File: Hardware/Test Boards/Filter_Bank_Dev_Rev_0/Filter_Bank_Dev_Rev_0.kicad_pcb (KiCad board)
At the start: 2 copper layers, 50 x 50 mm, 24 parts, among them J1 USB_B_Micro, J2 RF IN, J3 RF OUT, SW1 KAE02LGGR, U1 PE42440, U2 74AHC1G04, U3 AMS1117-3.3, U4 PE42440

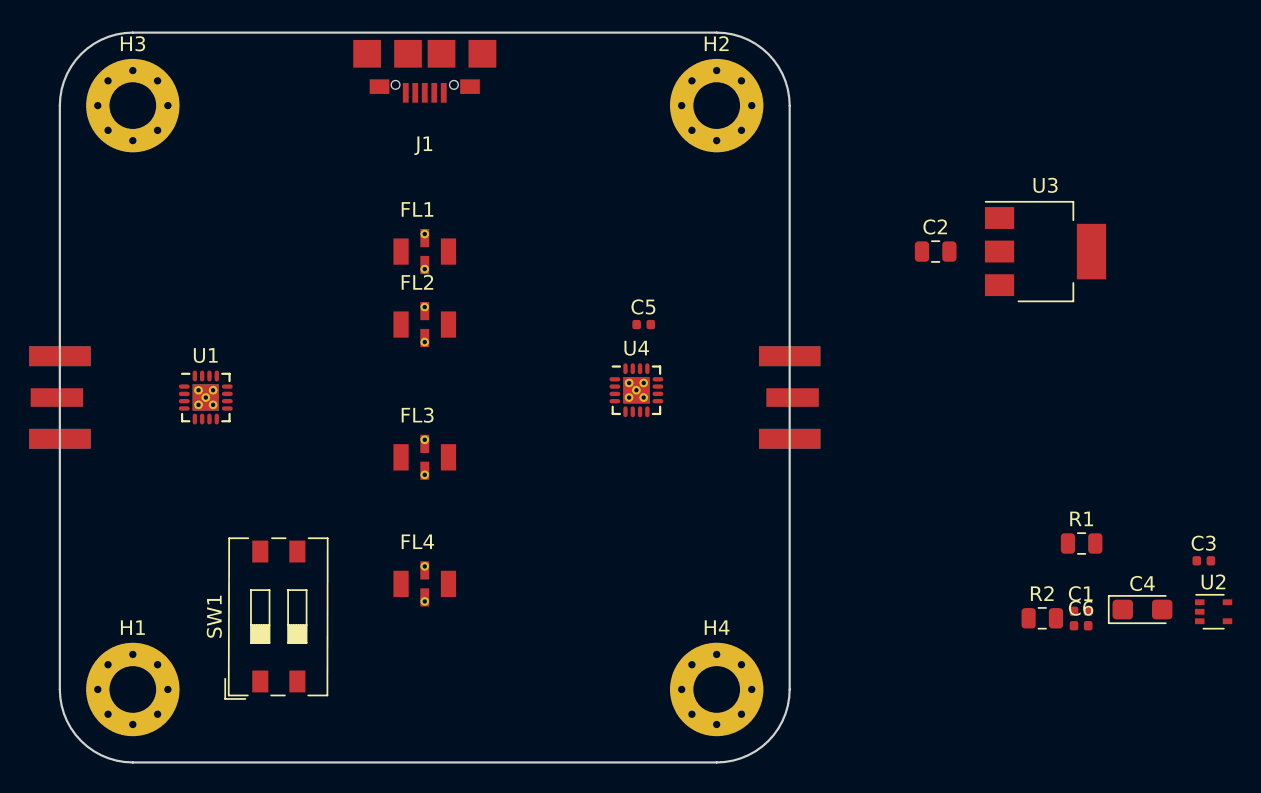
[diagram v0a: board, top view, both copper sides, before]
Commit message: Filter Bank layout finished
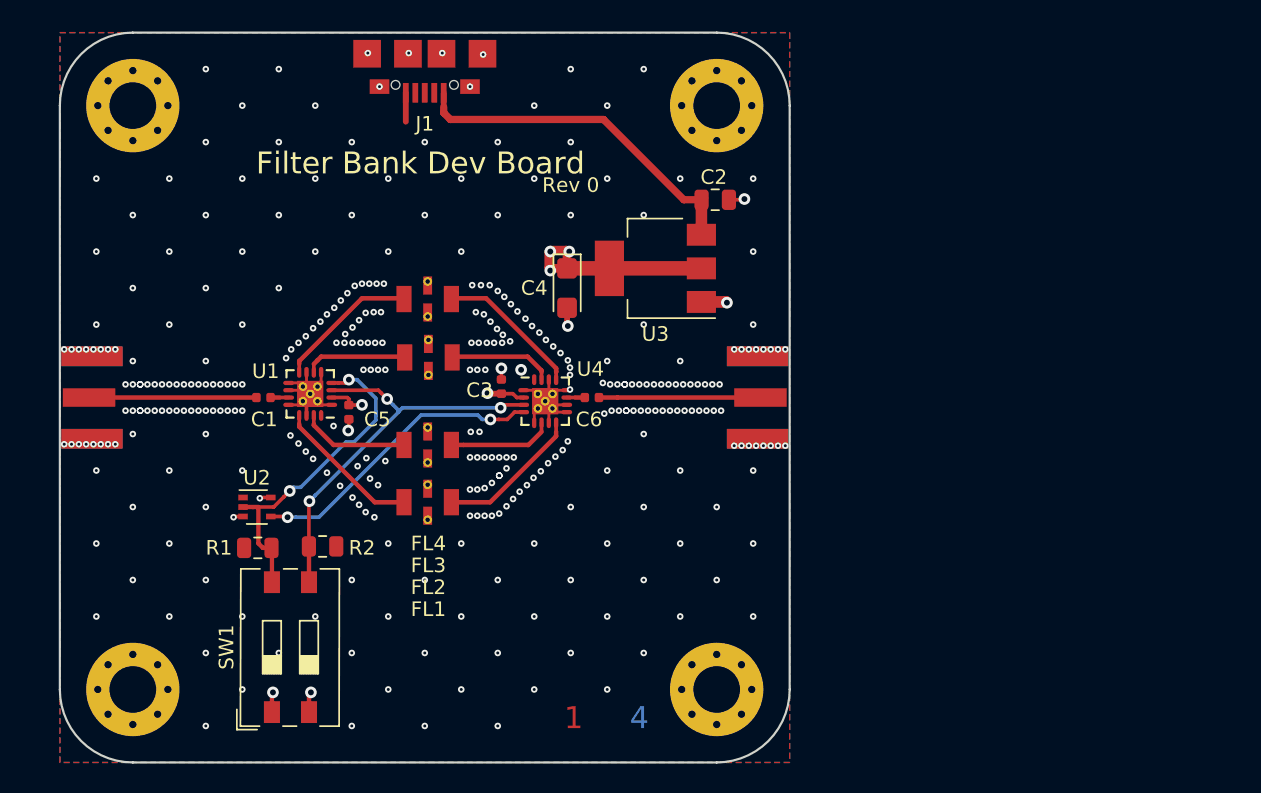
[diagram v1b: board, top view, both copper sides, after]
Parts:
- added G***: LOGO, VNA_Footprints:OSHW_Logo_3.6x3.6_F.Mask, F.Cu at (126.2, 86.8)
- added REF**: Board Title, VNA_Footprints:BoardTitle, F.Cu at (118.7, 45.7)
- added REF**: 4LayerCheck, VNA_Footprints:4LayerCheck, F.Cu at (132.7, 87.0)
- added REF**: Josh Details, VNA_Footprints:JoshDetails, B.Cu at (131.2, 82.5)
- FL3: value Filter_LFCN-400D+ -> Filter_LFCN-1000+
- FL4: value Filter_LFCN-1000+ -> Filter_LFCN-400D+
- U1, U4: footprint Package_DFN_QFN:QFN-16-1EP_3x3mm_P0.5mm_EP2.7x2.7mm_ThermalVias -> VNA_Footprints:QFN-16-1EP_3x3mm_P0.5mm_EP2.7x2.7mm_ThermalVias
- moved U2 65.9 mm to (108.5, 72.5)
- moved C1 57.9 mm to (109.0, 65.0), turned to 180 degrees
- moved R1 56.4 mm to (108.6, 75.3), turned to 180 degrees
- moved C3 49.6 mm to (125.2, 64.2), turned to 270 degrees
- moved R2 49.6 mm to (113.0, 75.2)
- moved J3 47.8 mm to (142.8, 65.0), turned to 0 degrees
- moved J2 47.8 mm to (97.2, 65.0), turned to 180 degrees
- moved C4 45.2 mm to (129.8, 57.5), turned to 270 degrees
- moved C6 37.0 mm to (131.4, 65.0), turned to 180 degrees
- moved U3 26.7 mm to (135.8, 56.1), turned to 180 degrees
- moved C5 21.1 mm to (114.8, 66.0), turned to 90 degrees
- moved FL4 19.5 mm to (120.2, 58.2)
- moved FL1 17.2 mm to (120.2, 72.2)
- moved C2 15.5 mm to (139.9, 51.5)
- moved FL2 8.25 mm to (120.2, 68.2)
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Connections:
- FL1 pad 3: /SW_2_RF_1 -> /SW_2_RF_3
- FL2 pad 3: /SW_2_RF_2 -> /SW_2_RF_4
- FL3 pad 1: /SW_1_RF_3 -> /SW_1_RF_4
- FL3 pad 3: /SW_2_RF_3 -> /SW_2_RF_2
- FL4 pad 1: /SW_1_RF_4 -> /SW_1_RF_3
- FL4 pad 3: /SW_2_RF_4 -> /SW_2_RF_1
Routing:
- net GND: track 0.00 -> 30.2 mm, vias 0 -> 339
- net /SW_1_CTRL_2: track 0.00 -> 28.2 mm, vias 0 -> 3
- net +5V: track 0.00 -> 24.2 mm
- net /SW_1_CTRL_1: track 0.00 -> 23.2 mm, vias 0 -> 2
- net +3V3: track 0.00 -> 22.8 mm, vias 0 -> 8
- net /SW_2_CTRL_1: track 0.00 -> 20.8 mm, vias 0 -> 2
- net Net-(C1-Pad2): track 0.00 -> 11.5 mm
- net Net-(C6-Pad1): track 0.00 -> 11.1 mm
- net /SW_1_RF_1: track 0.00 -> 10.1 mm
- net /SW_2_RF_3: track 0.00 -> 9.97 mm
- net /SW_2_RF_1: track 0.00 -> 9.94 mm
- net /SW_1_RF_3: track 0.00 -> 9.73 mm
- net /SW_1_RF_2: track 0.00 -> 7.41 mm
- net /SW_2_RF_2: track 0.00 -> 7.19 mm
- net /SW_2_RF_4: track 0.00 -> 7.17 mm
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- added copper zone on F.Cu, net +3V3
- added copper zone on In2.Cu, net +3V3
- added copper zone on B.Cu, net GND
- added copper zone on F.Cu, net GND
- added copper zone on In1.Cu, net GND
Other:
- copper layers 2 -> 4
- net class Default: clearance 0.2 -> 0.1
- net class RF added: clearance 0.1, trace_width 0.31, via_dia 0.45, via_drill 0.2
- rule trace_clearance: 0.2 -> 0.1
- rule trace_min: 0.2 -> 0.127
- rule via_min_drill: 0.3 -> 0.2
- rule via_min_size: 0.4 -> 0.45
